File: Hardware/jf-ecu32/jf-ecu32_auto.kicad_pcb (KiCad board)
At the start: 2 copper layers, 72.5 x 48.3 mm, 63 parts, among them J1 GAZ, J10 k, J11 RPM, J12 S.PORT, J13 PPM/PWM, J14 PUMP1, J15 PUMP1, J16 PPM/PWM, J17 PUMP2, J18 PUMP2, J2 AUX, J3 PPM/PWM, J4 STARTER, J5 GLOW, J6 VANNE KEROSTART, J7 VANNE KERO, J8 BATTERY 2S/3S, J9 STARTER, Q1 AO3400A, Q2 QM6006D, Q3 AO3400A, Q4 QM6006D, Q5 QM6006D, Q6 QM6006D, U1 ESP32-DevKitC, U2 4050, U3 MAX31855KASA, U4 AMS1117-3.3, U5 4050

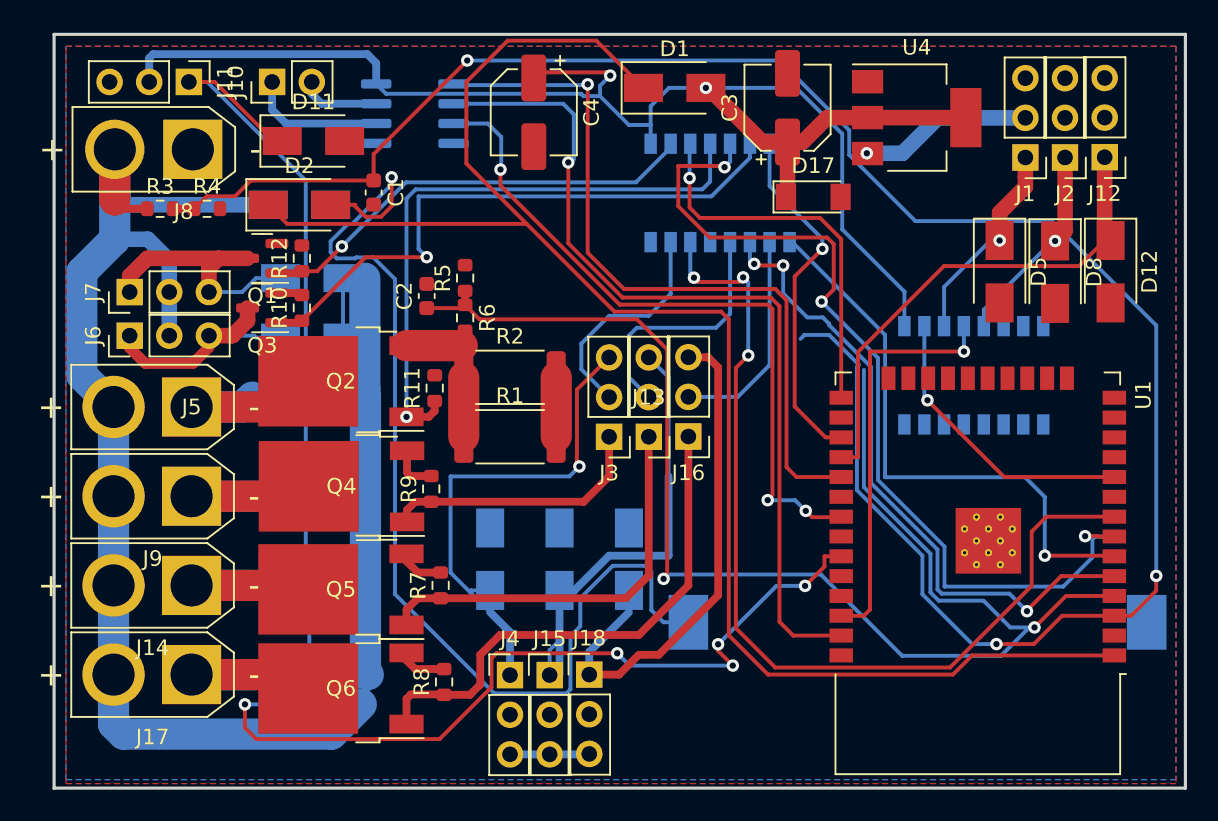
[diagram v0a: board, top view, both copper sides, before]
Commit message: pcb
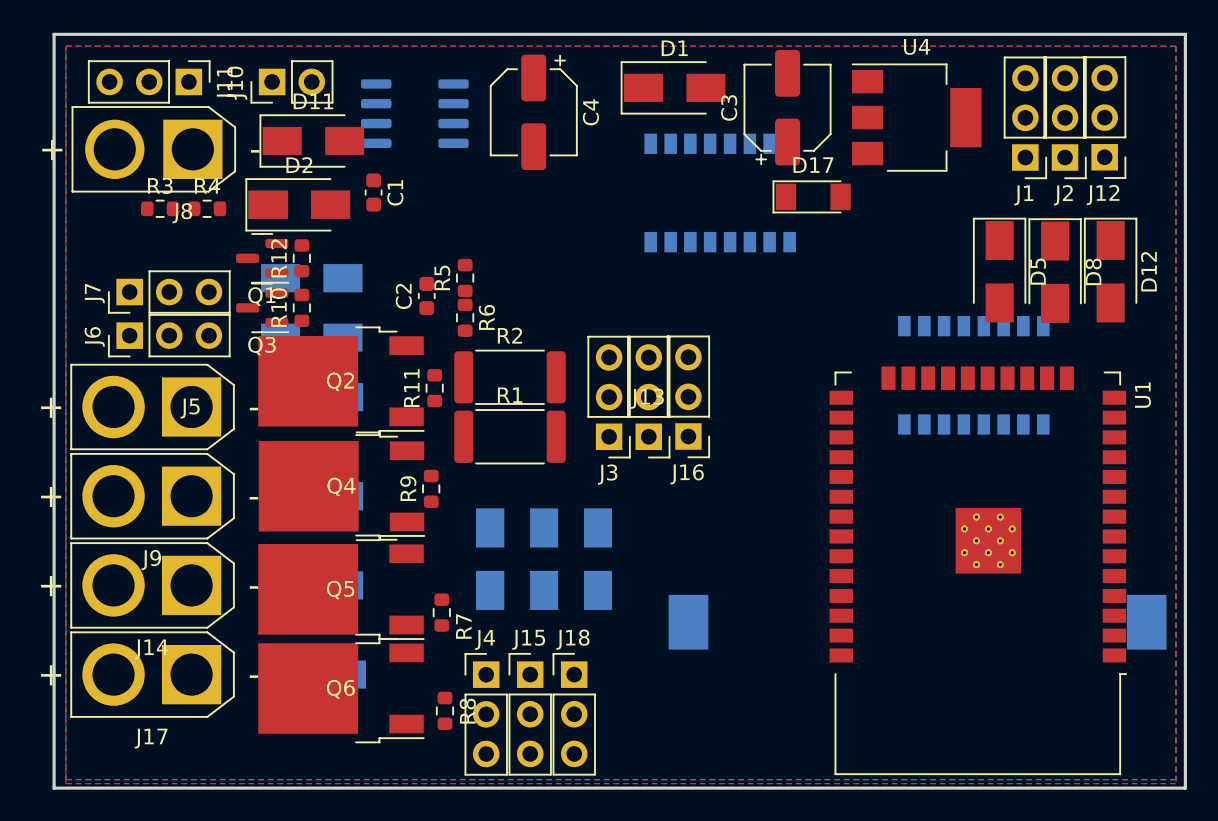
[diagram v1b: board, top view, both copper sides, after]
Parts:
- moved D16 1.98 mm to (48.8, 183.7)
- moved R8 1.85 mm to (39.0, 193.5)
- moved R7 1.74 mm to (38.8, 187.2)
- moved J4 1.52 mm to (41.7, 191.1)
- moved J15 1.24 mm to (44.5, 191.1)
- moved D14 0.99 mm to (45.4, 183.7)
- moved J18 0.97 mm to (47.3, 191.1)
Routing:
- net VBAT_ADC: track 131.7 -> 0.00 mm, vias 3 -> 0
- net +BATT: track 118.8 -> 0.00 mm
- net RPM: track 104.1 -> 0.00 mm, vias 5 -> 0
- net V_CPU: track 103.4 -> 0.00 mm
- net +3.3V: track 95.8 -> 0.00 mm, vias 2 -> 0
- net GLOW_CURRENT: track 88.4 -> 0.00 mm, vias 2 -> 0
- net Net-(BT1-Pad1): track 68.9 -> 0.00 mm, vias 1 -> 0
- net PPM_STARTER_3.3: track 60.0 -> 0.00 mm, vias 3 -> 0
- net PWM_GLOW_3.3: track 59.2 -> 0.00 mm, vias 3 -> 0
- net CS: track 56.2 -> 0.00 mm, vias 1 -> 0
- net CLK: track 47.9 -> 0.00 mm, vias 1 -> 0
- net MISO: track 44.8 -> 0.00 mm, vias 3 -> 0
- net PPM_PWM_PUMP1_3.3: track 41.9 -> 0.00 mm, vias 3 -> 0
- net PWM_GLOW: track 38.9 -> 0.00 mm, vias 1 -> 0
- net PWM_KEROSTART: track 38.6 -> 0.00 mm, vias 1 -> 0
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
